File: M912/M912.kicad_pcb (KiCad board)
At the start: 2 copper layers, 80 x 15 mm, 7 parts, among them J1 Conn_01x04

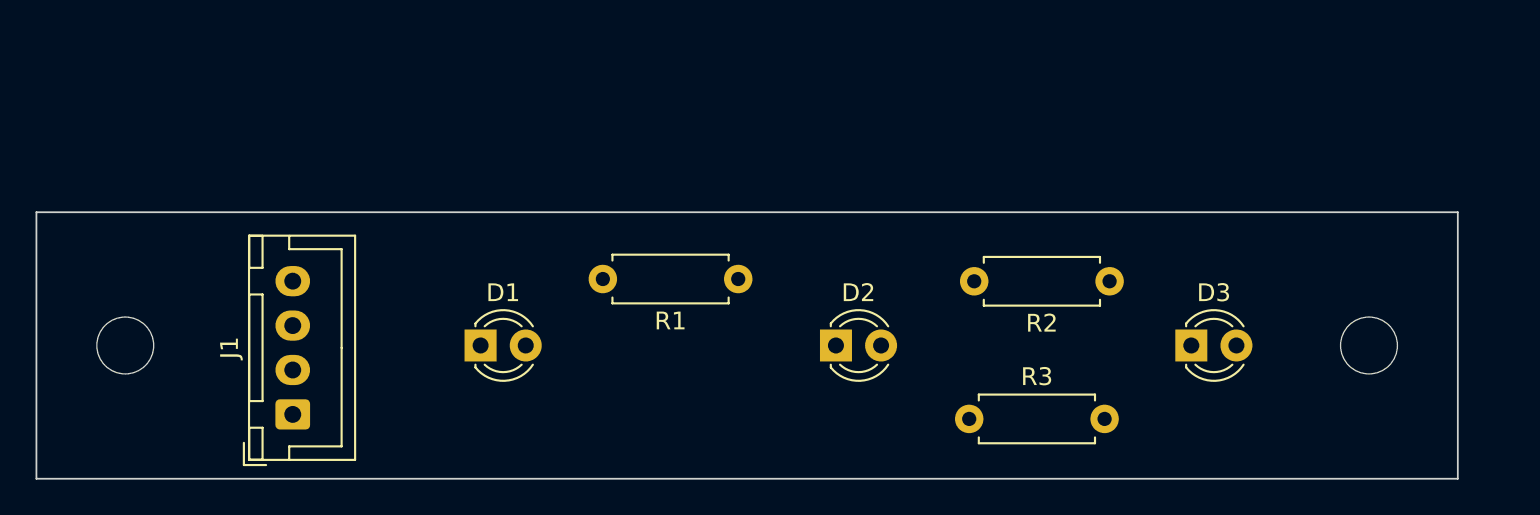
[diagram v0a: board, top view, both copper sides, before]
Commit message: 1st Release
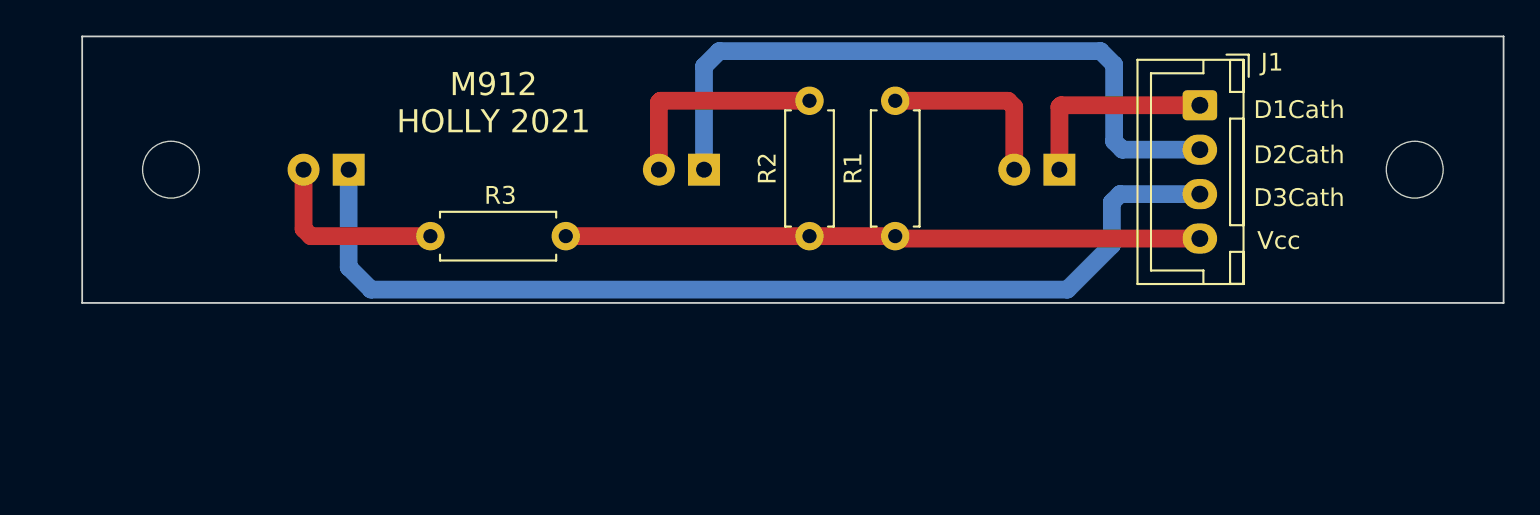
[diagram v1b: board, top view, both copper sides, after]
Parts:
- D1, D2, D3: moved to B.Cu
- moved J1 53.9 mm to (165.5, 94.0), turned to 270 degrees
- moved D3 48.4 mm to (117.6, 97.6), turned to 180 degrees
- moved D1 34.0 mm to (157.6, 97.6), turned to 180 degrees
- moved R3 24.9 mm to (129.8, 101.3), turned to 180 degrees
- moved R2 17.1 mm to (143.5, 101.3), turned to 90 degrees
- moved D2 12.4 mm to (137.6, 97.6), turned to 180 degrees
- moved R1 9.16 mm to (148.3, 101.3), turned to 90 degrees
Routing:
- net Net-(D3-Pad1): track 0.00 -> 57.6 mm
- net Net-(D2-Pad1): track 0.00 -> 38.9 mm
- net Net-(J1-Pad4): track 0.00 -> 35.7 mm
- net Net-(D2-Pad2): track 0.00 -> 12.3 mm
- net Net-(D1-Pad1): track 0.00 -> 11.5 mm
- net Net-(D3-Pad2): track 0.00 -> 10.6 mm
- net Net-(D1-Pad2): track 0.00 -> 10.4 mm
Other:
- board text added: "Anod"
- board text added: "Cath"
- board text added: "D1Cath"
- board text added: "D2Cath"
- board text added: "D3Cath"
- board text added: "M912 HOLLY 2021"
- board text added: "Vcc"
